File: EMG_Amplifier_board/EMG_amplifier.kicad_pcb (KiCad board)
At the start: 2 copper layers, 50 x 28 mm, 54 parts, among them J1 Conn_01x04_Socket, J2 Conn_01x04_Pin, J3 Conn_01x06_Pin, J4 Conn_01x06_Socket, J7 Conn_01x06_Pin, U1 LPV821DBVR, U2 INA333xxDGK, U3 LPV821DBVR, U5 LPV821DBVR, U6 LPV821DBVR, U7 TPD2E001DRLR, U8 TLV8542DR

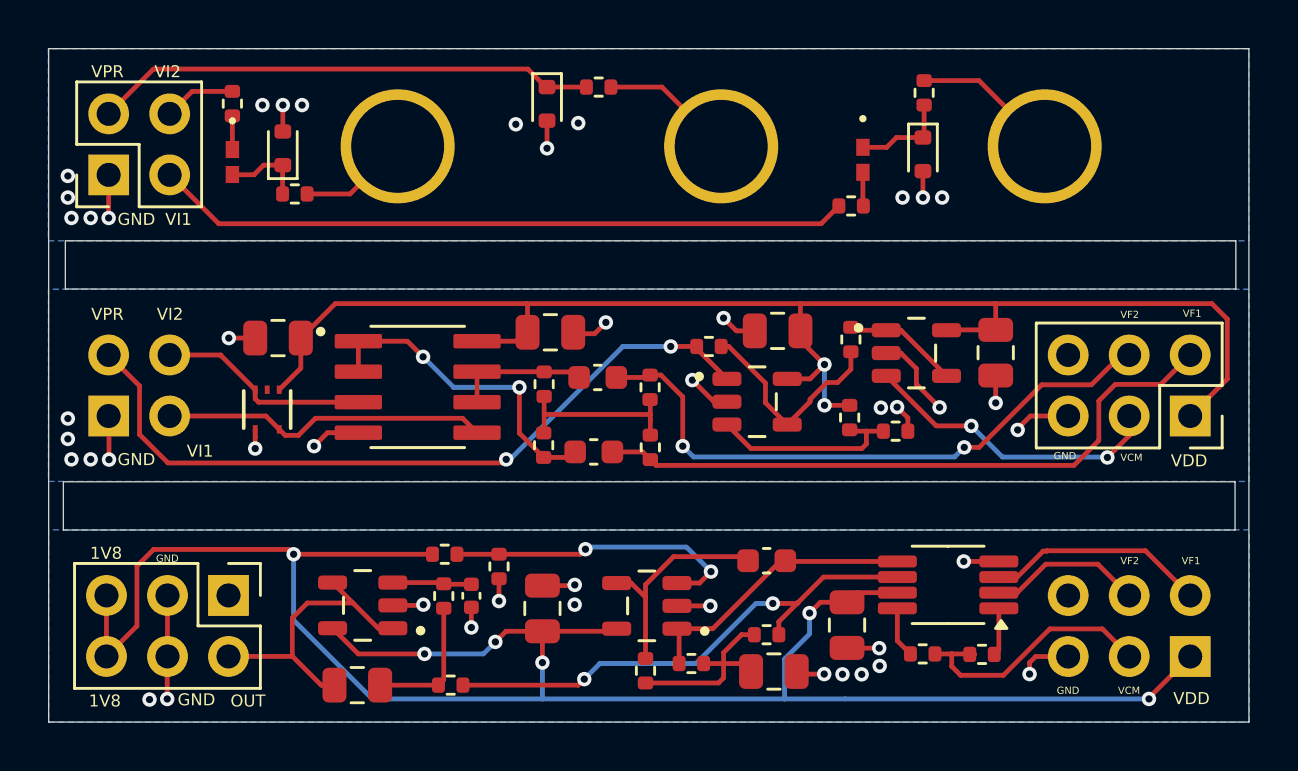
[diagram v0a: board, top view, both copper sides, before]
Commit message: aesthetics
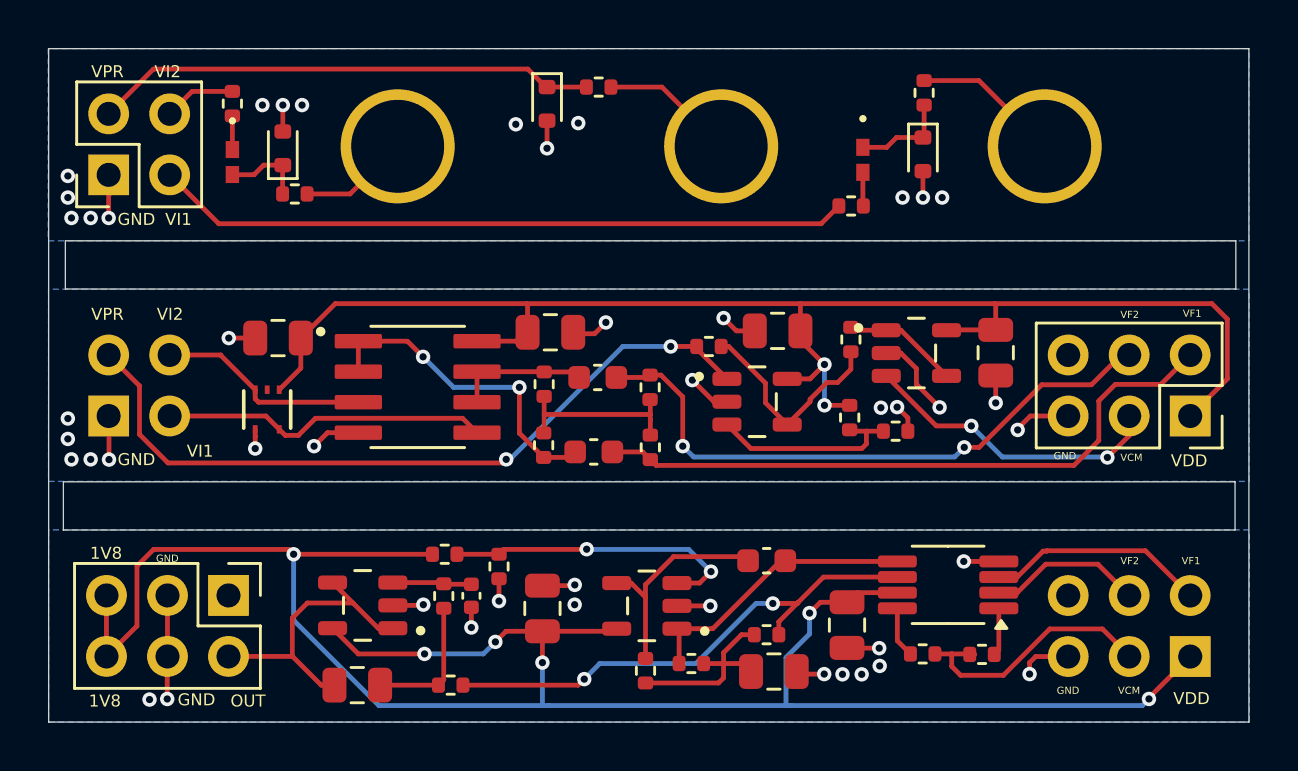
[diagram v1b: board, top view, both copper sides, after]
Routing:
- net +1V8: track 85.3 -> 86.1 mm
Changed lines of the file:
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@@
 	)
 	(segment
-		(start 34.35 32.8406)
-		(end 34.1406 33.05)
-		(width 0.2)
-		(layer "F.Cu")
-		(net 30)
-	)
-	(segment
-		(start 34.1406 33.05)
+		(start 34.4 32.8406)
+		(end 34.3906 32.85)
+		(width 0.2)
+		(layer "F.Cu")
+		(net 30)
+	)
+	(segment
+		(start 34.3906 32.85)
+		(end 30.95 32.85)
+		(width 0.2)
+		(layer "F.Cu")
+		(net 30)
+	)
+	(segment
+		(start 30.95 32.85)
 		(end 30.75 33.05)
 		(width 0.2)
@@
 	)
 	(via
-		(at 34.35 32.8406)
-		(size 0.6)
-		(drill 0.3)
-		(layers "F.Cu" "B.Cu")
-		(net 30)
-	)
-	(segment
-		(start 34.4406 32.75)
-		(end 34.35 32.8406)
-		(width 0.2)
-		(layer "B.Cu")
-		(net 30)
-	)
-	(segment
-		(start 39.575 33.775)
-		(end 38.55 32.75)
-		(width 0.2)
-		(layer "B.Cu")
-		(net 30)
-	)
-	(segment
-		(start 38.55 32.75)
-		(end 34.4406 32.75)
+		(at 34.4 32.8406)
+		(size 0.6)
+		(drill 0.3)
+		(layers "F.Cu" "B.Cu")
+		(net 30)
+	)
+	(segment
+		(start 34.4 32.8406)
+		(end 34.4094 32.85)
+		(width 0.2)
+		(layer "B.Cu")
+		(net 30)
+	)
+	(segment
+		(start 34.4094 32.85)
+		(end 38.65 32.85)
+		(width 0.2)
+		(layer "B.Cu")
+		(net 30)
+	)
+	(segment
+		(start 38.65 32.85)
+		(end 39.575 33.775)
 		(width 0.2)
 		(layer "B.Cu")
@@
 	)
 	(segment
+		(start 22.2 35.7964)
+		(end 25.7536 39.35)
+		(width 0.2)
+		(layer "B.Cu")
+		(net 33)
+	)
+	(segment
+		(start 32.8338 39.35)
+		(end 42.9156 39.35)
+		(width 0.2)
+		(layer "B.Cu")
+		(net 33)
+	)
+	(segment
+		(start 42.9156 39.35)
+		(end 57.5352 39.35)
+		(width 0.2)
+		(layer "B.Cu")
+		(net 33)
+	)
+	(segment
+		(start 32.55 39.35)
+		(end 32.5582 39.3418)
+		(width 0.2)
+		(layer "B.Cu")
+		(net 33)
+	)
+	(segment
+		(start 30.1 37.2)
+		(end 30.6 36.7)
+		(width 0.2)
+		(layer "B.Cu")
+		(net 33)
+	)
+	(segment
+		(start 57.5352 39.35)
+		(end 57.8108 39.0744)
+		(width 0.2)
+		(layer "B.Cu")
+		(net 33)
+	)
+	(segment
+		(start 42.7 37.35)
+		(end 43.68 36.37)
+		(width 0.2)
+		(layer "B.Cu")
+		(net 33)
+	)
+	(segment
+		(start 22.2 33.05)
+		(end 22.2 35.7964)
+		(width 0.2)
+		(layer "B.Cu")
+		(net 33)
+	)
+	(segment
+		(start 32.5582 39.3418)
+		(end 32.5582 37.562)
+		(width 0.2)
+		(layer "B.Cu")
+		(net 33)
+	)
+	(segment
+		(start 27.65 37.2)
+		(end 30.1 37.2)
+		(width 0.2)
+		(layer "B.Cu")
+		(net 33)
+	)
+	(segment
 		(start 43.68 36.37)
 		(end 43.68 35.5)
@@
 	)
 	(segment
-		(start 42.64 39.0744)
-		(end 42.64 37.41)
-		(width 0.2)
-		(layer "B.Cu")
-		(net 33)
-	)
-	(segment
-		(start 22.2 33.05)
-		(end 22.2 35.7964)
-		(width 0.2)
-		(layer "B.Cu")
-		(net 33)
-	)
-	(segment
-		(start 32.5582 39.0744)
-		(end 42.64 39.0744)
-		(width 0.2)
-		(layer "B.Cu")
-		(net 33)
-	)
-	(segment
-		(start 25.478 39.0744)
-		(end 32.5582 39.0744)
-		(width 0.2)
-		(layer "B.Cu")
-		(net 33)
-	)
-	(segment
-		(start 30.1 37.2)
-		(end 30.6 36.7)
-		(width 0.2)
-		(layer "B.Cu")
-		(net 33)
-	)
-	(segment
-		(start 42.64 37.41)
-		(end 43.68 36.37)
-		(width 0.2)
-		(layer "B.Cu")
-		(net 33)
-	)
-	(segment
-		(start 42.64 39.0744)
-		(end 45.16 39.0744)
-		(width 0.2)
-		(layer "B.Cu")
-		(net 33)
-	)
-	(segment
-		(start 57.8108 39.0744)
-		(end 45.16 39.0744)
-		(width 0.2)
-		(layer "B.Cu")
-		(net 33)
-	)
-	(segment
-		(start 32.5582 39.0744)
-		(end 32.5582 37.562)
-		(width 0.2)
-		(layer "B.Cu")
-		(net 33)
-	)
-	(segment
-		(start 22.2 35.7964)
-		(end 25.478 39.0744)
-		(width 0.2)
-		(layer "B.Cu")
-		(net 33)
-	)
-	(segment
-		(start 27.65 37.2)
-		(end 30.1 37.2)
-		(width 0.2)
-		(layer "B.Cu")
+		(start 42.7 39.35)
+		(end 42.7 37.35)
+		(width 0.2)
+		(layer "B.Cu")
+		(net 33)
+	)
+	(segment
+		(start 25.7536 39.35)
+		(end 32.8338 39.35)
+		(width 0.2)
+		(layer "B.Cu")
